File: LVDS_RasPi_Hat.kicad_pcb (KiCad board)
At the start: 2 copper layers, 72 x 67 mm, 37 parts, among them J1 Raspberry_Pi_2_3, J2 RJHSE508002, J3 Conn_Coaxial_Small, J4 Conn_Coaxial_Small, J5 Conn_Coaxial_Small, J6 Conn_Coaxial_Small, J7 Conn_02x16, U1 SN65MLVD206BD, U2 SN65MLVD206BD, U3 SN65MLVD206BD, U4 SN65MLVD206BD, U5 SN65LVDT348D, U6 SN65LVDT348D, U7 SN65LVDT348D, U8 SN65LVDT348D, U9 SN65LVDT348D

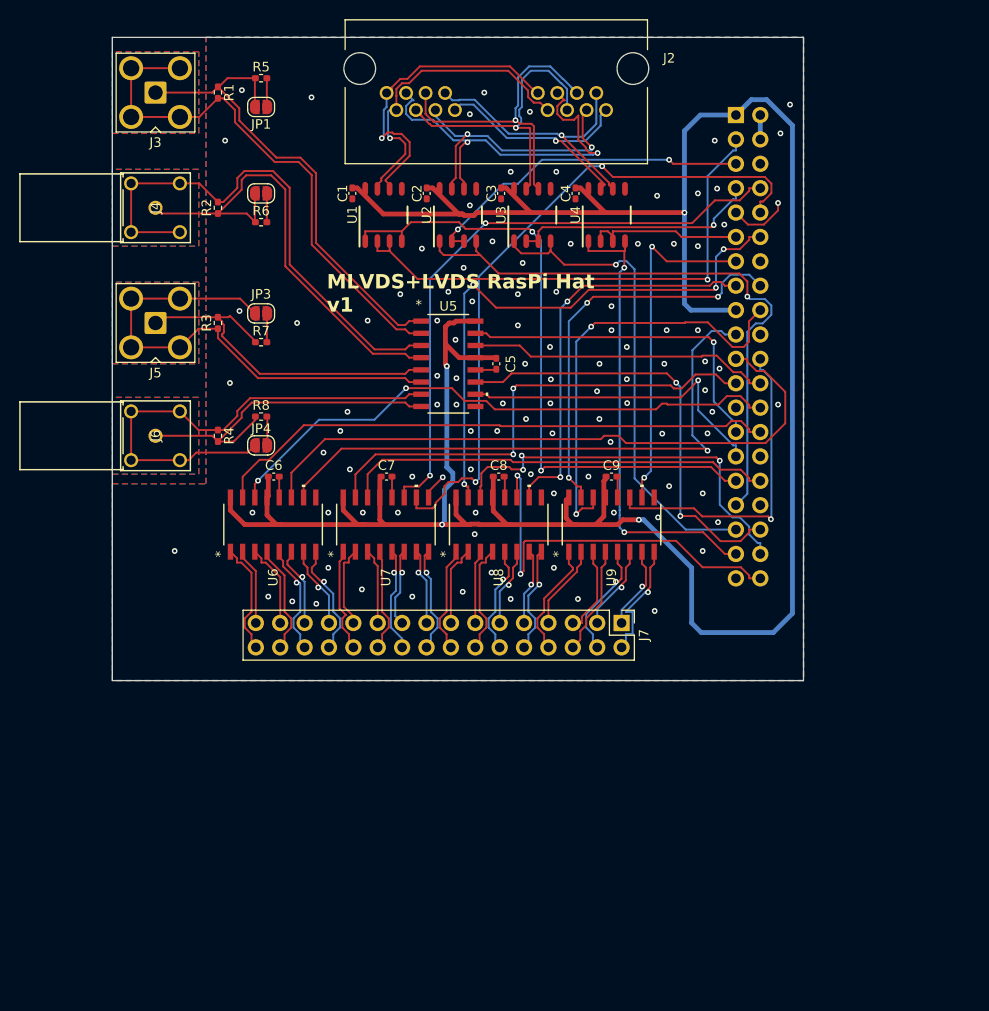
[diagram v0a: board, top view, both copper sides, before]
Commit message: v2
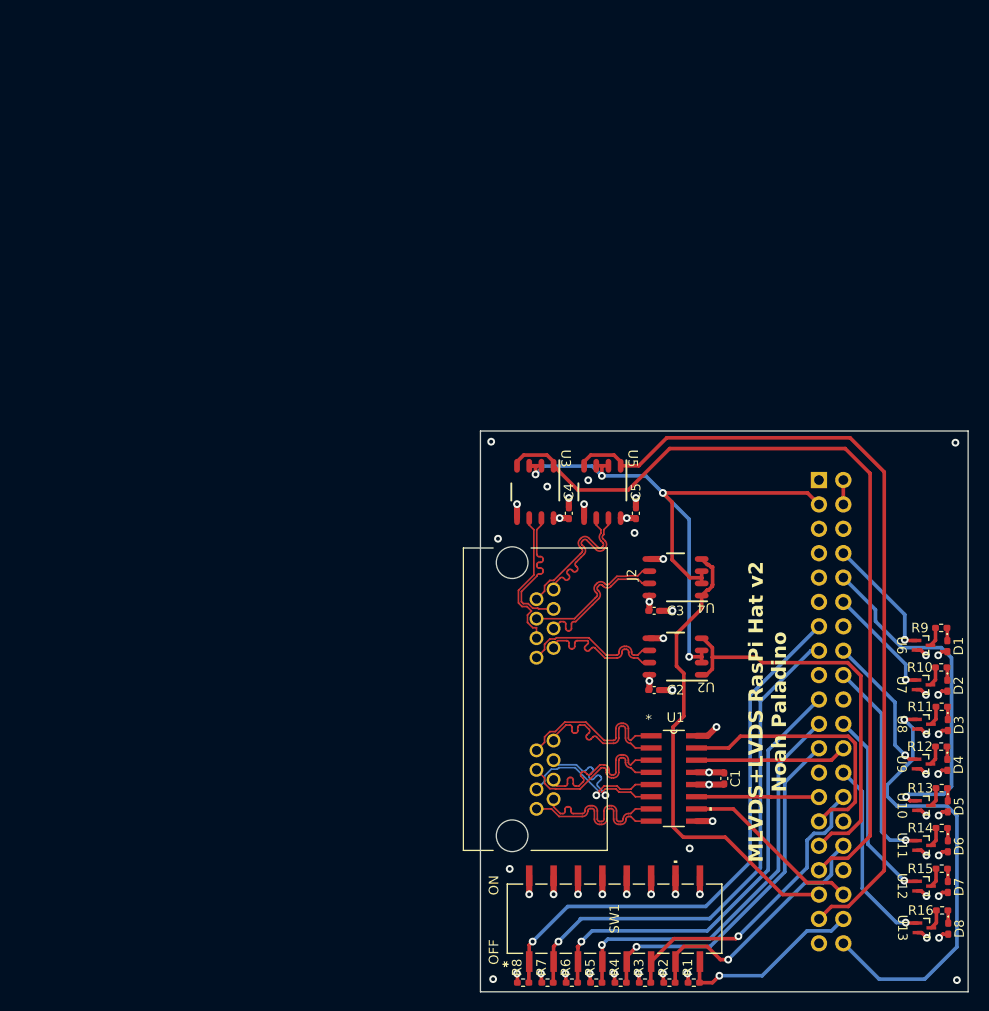
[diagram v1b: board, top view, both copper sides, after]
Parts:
- removed C6, C7, C8, C9: C100n, Capacitor_SMD:C_0402_1005Metric_Pad0.74x0.62mm_HandSolder
- removed J3, J5: Conn_Coaxial_Small, Connector_Coaxial:SMA_Amphenol_901-143_Horizontal
- removed J4, J6: Conn_Coaxial_Small, EPL_00_250_NTN:CONN_EPK.00.250.NTN_LMO
- removed J7: Conn_02x16, Connector_PinHeader_2.54mm:PinHeader_2x16_P2.54mm_Vertical
- removed JP1, JP2, JP3, JP4: SolderJumper_2_Open, Jumper:SolderJumper-2_P1.3mm_Open_RoundedPad1.0x1.5mm
- added D1: LED, LED_SMD:LED_0402_1005Metric_Pad0.77x0.64mm_HandSolder, F.Cu at (112.1, 85.9)
- added D2: LED, LED_SMD:LED_0402_1005Metric_Pad0.77x0.64mm_HandSolder, F.Cu at (112.1, 90.0)
- added D3: LED, LED_SMD:LED_0402_1005Metric_Pad0.77x0.64mm_HandSolder, F.Cu at (112.2, 94.1)
- added D4: LED, LED_SMD:LED_0402_1005Metric_Pad0.77x0.64mm_HandSolder, F.Cu at (112.1, 98.3)
- added D5: LED, LED_SMD:LED_0402_1005Metric_Pad0.77x0.64mm_HandSolder, F.Cu at (112.2, 102.6)
- added D6: LED, LED_SMD:LED_0402_1005Metric_Pad0.77x0.64mm_HandSolder, F.Cu at (112.2, 106.8)
- added D7: LED, LED_SMD:LED_0402_1005Metric_Pad0.77x0.64mm_HandSolder, F.Cu at (112.2, 111.0)
- added D8: LED, LED_SMD:LED_0402_1005Metric_Pad0.77x0.64mm_HandSolder, F.Cu at (112.2, 115.3)
- added R10: R470, Resistor_SMD:R_0402_1005Metric_Pad0.72x0.64mm_HandSolder, F.Cu at (111.5, 88.1)
- added R11: R470, Resistor_SMD:R_0402_1005Metric_Pad0.72x0.64mm_HandSolder, F.Cu at (111.5, 92.2)
- added R12: R470, Resistor_SMD:R_0402_1005Metric_Pad0.72x0.64mm_HandSolder, F.Cu at (111.5, 96.4)
- added R13: R470, Resistor_SMD:R_0402_1005Metric_Pad0.72x0.64mm_HandSolder, F.Cu at (111.5, 100.7)
- added R14: R470, Resistor_SMD:R_0402_1005Metric_Pad0.72x0.64mm_HandSolder, F.Cu at (111.6, 104.9)
- added R15: R470, Resistor_SMD:R_0402_1005Metric_Pad0.72x0.64mm_HandSolder, F.Cu at (111.6, 109.1)
- added R16: R470, Resistor_SMD:R_0402_1005Metric_Pad0.72x0.64mm_HandSolder, F.Cu at (111.6, 113.4)
- added R9: R470, Resistor_SMD:R_0402_1005Metric_Pad0.72x0.64mm_HandSolder, F.Cu at (111.5, 84.0)
- added SW1: SW_DIP_x08, 219_8LPST:219-8LPST_CTS-M, F.Cu at (77.5, 114.3)
- added U10: DMN26D0UT-7, DMN26D0UT_7:DMN26D0UT-7_PER, F.Cu at (109.7, 102.5)
- added U11: DMN26D0UT-7, DMN26D0UT_7:DMN26D0UT-7_PER, F.Cu at (109.7, 106.7)
- added U12: DMN26D0UT-7, DMN26D0UT_7:DMN26D0UT-7_PER, F.Cu at (109.7, 110.9)
- added U13: DMN26D0UT-7, DMN26D0UT_7:DMN26D0UT-7_PER, F.Cu at (109.7, 115.3)
- R1, R2, R3, R4: value R100 -> R4.7k
- R5, R6, R7, R8: value R50 -> R4.7k
- U1: value SN65MLVD206BD -> SN65LVDT348D; footprint SN65MLVD206BD:D0008A_N -> SN65LVDT348D:D16
- U5: value SN65LVDT348D -> SN65MLVD206BD; footprint SN65LVDT348D:D16-M -> SN65MLVD206BD:D0008A_N
- U6, U7, U8, U9: value SN65LVDT348D -> DMN26D0UT-7; footprint SN65LVDT348D:D16-M -> DMN26D0UT_7:DMN26D0UT-7_PER
- moved R1 105.1 mm to (85.7, 121.0), turned to 0 degrees
- moved R5 100.5 mm to (75.6, 121.0)
- moved R2 93.4 mm to (83.2, 121.0), turned to 0 degrees
- moved R6 85.6 mm to (73.0, 121.0)
- moved R3 81.9 mm to (80.6, 121.0), turned to 0 degrees
- moved R7 73.1 mm to (70.5, 121.0)
- moved C1 72.2 mm to (88.9, 99.7)
- moved R4 70.7 mm to (78.1, 121.0), turned to 0 degrees
- moved U6 68.9 mm to (109.7, 85.8), turned to -90 degrees
- moved U1 66.0 mm to (83.6, 99.7), turned to 0 degrees
- moved J2 65.7 mm to (66.8, 91.4), turned to -90 degrees
- moved R8 65.0 mm to (67.9, 121.0)
- moved U7 58.4 mm to (109.7, 89.9), turned to -90 degrees
- moved C2 56.9 mm to (81.6, 90.5), turned to 0 degrees
- moved U2 51.3 mm to (83.8, 87.0), turned to 180 degrees
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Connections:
- J1 pad 10: /TRIGGER7 -> /CONFIG12
- J1 pad 11: /TS_BUS_SEL3 -> unconnected-(J1-GPIO17-Pad11)
- J1 pad 12: /TRIGGER8 -> /CONFIG9
- J1 pad 13: /TRIGGER15 -> /CONFIG7
- J1 pad 15: /TRIGGER11 -> /CONFIG6
- J1 pad 16: /TRIGGER12 -> /CONFIG11
- J1 pad 18: /TRIGGER13 -> /CONFIG13
- J1 pad 19: /TRIGGER3 -> /CONFIG5
- J1 pad 21: /TRIGGER2 -> /CONFIG4
- J1 pad 22: /TRIGGER14 -> /CONFIG14
- J1 pad 23: /TRIGGER4 -> /CONFIG3
- J1 pad 24: /NIM1 -> /NIM2
- J1 pad 26: /TRIGGER1 -> /CONFIG15
- J1 pad 27: /NIM0 -> /NIM1
- J1 pad 28: /TRIGGER0 -> /CONFIG2
- J1 pad 3: /TS_BUS_SEL0 -> /TS_BUS_SEL
- J1 pad 32: /TRIGGER5 -> /CONFIG1
- J1 pad 36: /NIM2 -> /NIM0
- J1 pad 38: /TRIGGER9 -> /CONFIG0
- J1 pad 40: /TRIGGER10 -> /CONFIG10
- J1 pad 5: /TS_BUS_SEL1 -> unconnected-(J1-SCL/GPIO3-Pad5)
- J1 pad 7: /TS_BUS_SEL2 -> unconnected-(J1-GCLK0/GPIO4-Pad7)
- J1 pad 8: /TRIGGER6 -> /CONFIG8
- J2 pad 2_1: /Trigger Interface/D1+ -> /Trigger Interface/S1-
- J2 pad 2_2: /Trigger Interface/D1- -> /Trigger Interface/S1+
- J2 pad 2_3: /Trigger Interface/D2+ -> /Trigger Interface/S2-
- J2 pad 2_4: /Trigger Interface/D3- -> /Trigger Interface/S3+
- J2 pad 2_5: /Trigger Interface/D3+ -> /Trigger Interface/S3-
- J2 pad 2_6: /Trigger Interface/D2- -> /Trigger Interface/S2+
- J2 pad 2_7: /Trigger Interface/D4+ -> /Trigger Interface/S4-
- J2 pad 2_8: /Trigger Interface/D4- -> /Trigger Interface/S4+
- R1 pad 1: /Trigger Interface/NIM1- -> +3V3
- R1 pad 2: /Trigger Interface/NIM1+ -> /CONFIG0
- R2 pad 1: /Trigger Interface/NIM2- -> +3V3
- R2 pad 2: /Trigger Interface/NIM2+ -> /CONFIG1
- R3 pad 1: /Trigger Interface/NIM3+ -> +3V3
- R3 pad 2: /Trigger Interface/NIM3- -> /CONFIG2
- R4 pad 1: /Trigger Interface/NIM4+ -> +3V3
- R4 pad 2: /Trigger Interface/NIM4- -> /CONFIG3
- R5 pad 1: /Trigger Interface/NIM1- -> +3V3
- R5 pad 2: GND -> /CONFIG4
- R6 pad 1: /Trigger Interface/NIM2- -> +3V3
- R6 pad 2: GND -> /CONFIG5
- R7 pad 1: /Trigger Interface/NIM3- -> +3V3
- R7 pad 2: GND -> /CONFIG6
- R8 pad 1: /Trigger Interface/NIM4- -> +3V3
- R8 pad 2: GND -> /CONFIG7
- U1 pad 1: /TS_BUS0 -> /Trigger Interface/S4-
- U1 pad 2: /TS_BUS_SEL0 -> /Trigger Interface/S4+
- U1 pad 3: /TS_BUS_SEL0 -> /Trigger Interface/S3+
- U1 pad 4: /TS_BUS0 -> /Trigger Interface/S3-
- U1 pad 5: GND -> /Trigger Interface/S2-
- U1 pad 6: /Trigger Interface/D1+ -> /Trigger Interface/S2+
- U1 pad 7: /Trigger Interface/D1- -> /Trigger Interface/S1+
- U1 pad 8: +3V3 -> /Trigger Interface/S1-
- U2 pad 1: /TS_BUS1 -> /TS_BUS0
- U2 pad 2: /TS_BUS_SEL1 -> /TS_BUS_SEL
- U2 pad 3: /TS_BUS_SEL1 -> /TS_BUS_SEL
- U2 pad 4: /TS_BUS1 -> /TS_BUS0
- U2 pad 6: /Trigger Interface/D2+ -> /Trigger Interface/D1+
- U2 pad 7: /Trigger Interface/D2- -> /Trigger Interface/D1-
- U3 pad 1: /TS_BUS2 -> /TS_BUS1
- U3 pad 2: /TS_BUS_SEL2 -> /TS_BUS_SEL
- U3 pad 3: /TS_BUS_SEL2 -> /TS_BUS_SEL
- U3 pad 4: /TS_BUS2 -> /TS_BUS1
- U3 pad 6: /Trigger Interface/D3+ -> /Trigger Interface/D2+
- U3 pad 7: /Trigger Interface/D3- -> /Trigger Interface/D2-
- U4 pad 1: /TS_BUS3 -> /TS_BUS2
- U4 pad 2: /TS_BUS_SEL3 -> /TS_BUS_SEL
- U4 pad 3: /TS_BUS_SEL3 -> /TS_BUS_SEL
- U4 pad 4: /TS_BUS3 -> /TS_BUS2
- U4 pad 6: /Trigger Interface/D4+ -> /Trigger Interface/D3+
- U4 pad 7: /Trigger Interface/D4- -> /Trigger Interface/D3-
- U5 pad 1: /Trigger Interface/NIM1- -> /TS_BUS3
- U5 pad 2: /Trigger Interface/NIM1+ -> /TS_BUS_SEL
- U5 pad 3: /Trigger Interface/NIM2+ -> /TS_BUS_SEL
- U5 pad 4: /Trigger Interface/NIM2- -> /TS_BUS3
- U5 pad 5: /Trigger Interface/NIM3- -> GND
- U5 pad 6: /Trigger Interface/NIM3+ -> /Trigger Interface/D4+
- U5 pad 7: /Trigger Interface/NIM4+ -> /Trigger Interface/D4-
- U5 pad 8: /Trigger Interface/NIM4- -> +3V3
- U6 pad 1: /Trigger Interface/Trigger Signals/In0- -> /CONFIG8
- U6 pad 2: /Trigger Interface/Trigger Signals/In0+ -> GND
- U6 pad 3: /Trigger Interface/Trigger Signals/In1+ -> Net-(R9-Pad1)
- U7 pad 1: /Trigger Interface/Trigger Signals/In4- -> /CONFIG9
- U7 pad 2: /Trigger Interface/Trigger Signals/In4+ -> GND
- U7 pad 3: /Trigger Interface/Trigger Signals/In5+ -> Net-(R10-Pad1)
- U8 pad 1: /Trigger Interface/Trigger Signals/In8- -> /CONFIG10
- U8 pad 2: /Trigger Interface/Trigger Signals/In8+ -> GND
- U8 pad 3: /Trigger Interface/Trigger Signals/In9+ -> Net-(R11-Pad1)
- U9 pad 1: /Trigger Interface/Trigger Signals/In12- -> /CONFIG11
- U9 pad 2: /Trigger Interface/Trigger Signals/In12+ -> GND
- U9 pad 3: /Trigger Interface/Trigger Signals/In13+ -> Net-(R12-Pad1)
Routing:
- net +3V3: track 270.8 -> 28.5 mm, vias 4 -> 22
- net /TRIGGER7: track 70.6 -> 0.00 mm, vias 2 -> 0
- net /TS_BUS_SEL: track 0.00 -> 69.3 mm, vias 0 -> 4
- net /TRIGGER2: track 66.8 -> 0.00 mm
- net /TRIGGER6: track 63.3 -> 0.00 mm, vias 2 -> 0
- net /TRIGGER3: track 61.6 -> 0.00 mm, vias 1 -> 0
- net /TRIGGER1: track 60.4 -> 0.00 mm, vias 2 -> 0
- net /TRIGGER0: track 59.2 -> 0.00 mm
- net /TRIGGER8: track 58.8 -> 0.00 mm, vias 4 -> 0
- net /CONFIG7: track 0.00 -> 58.1 mm, vias 0 -> 1
- net /Trigger Interface/NIM1+: track 56.3 -> 0.00 mm
- net /Trigger Interface/NIM2+: track 55.7 -> 0.00 mm
- net /CONFIG6: track 0.00 -> 54.4 mm, vias 0 -> 1
- net /TS_BUS_SEL0: track 53.7 -> 0.00 mm, vias 1 -> 0
- net /Trigger Interface/NIM3+: track 52.5 -> 0.00 mm
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- added copper zone on In2.Cu, net +3V3
- added copper zone on In1.Cu, net GND
- added copper zone on In2.Cu, net GND
- removed copper zone on B.Cu, net /Trigger Interface/NIM1+
- removed copper zone on F.Cu, net /Trigger Interface/NIM1+
- removed copper zone on B.Cu, net /Trigger Interface/NIM2+
- removed copper zone on F.Cu, net /Trigger Interface/NIM2+
- removed copper zone on B.Cu, net /Trigger Interface/NIM3+
- removed copper zone on F.Cu, net /Trigger Interface/NIM3+
- removed copper zone on B.Cu, net /Trigger Interface/NIM4+
- removed copper zone on F.Cu, net /Trigger Interface/NIM4+
- removed copper zone on B.Cu, net GND
- removed copper zone on F.Cu, net GND
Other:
- board size 72 x 67 mm -> 50.8 x 58.4 mm
- copper layers 2 -> 4
- board text added: "MLVDS+LVDS RasPi Hat v${REVISION} Noah Paladino"
- board text removed: "MLVDS+LVDS RasPi Hat v1"
